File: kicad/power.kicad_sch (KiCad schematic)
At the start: 21 parts, among them U1 HT7533-1, U2 TLV62569DBV, U3 MCP6001T-E/OT

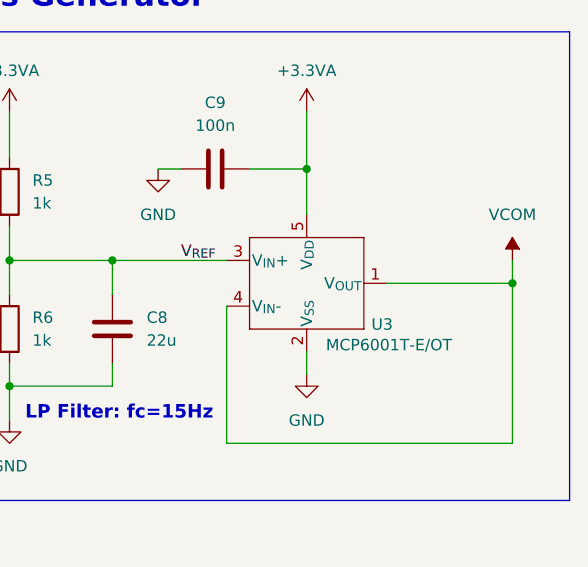
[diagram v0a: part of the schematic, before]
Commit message: Small update
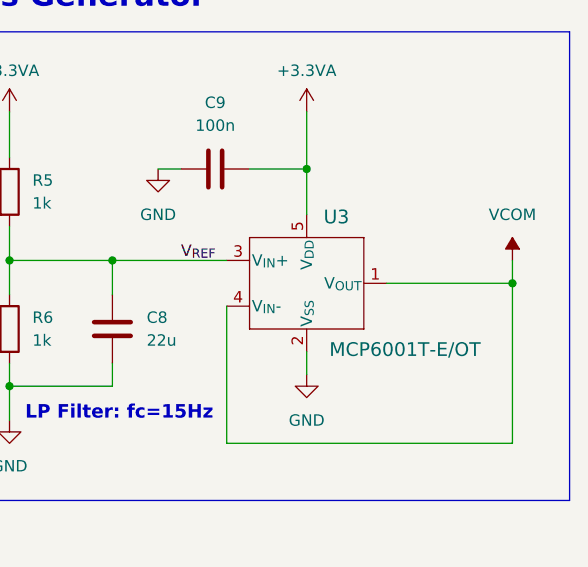
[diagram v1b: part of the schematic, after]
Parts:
- removed U3: MCP6001T-E/OT, SOT-23-5_MC_MCH, symbol bias_generator_ic:MCP6001T-E_OT
- added U3: MCP6001T-E/OT, SOT-23-5_MC_MCH, symbol bias_generator_microchip:MCP6001T-E_OT
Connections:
- net +3.3VA: now also U3.5 (V_{DD})
- net GND: now also U3.2 (V_{SS})
- net VCOM: now also U3.1 (V_{OUT}), U3.4 (V_{IN}-)
- net V_{REF}: now also U3.3 (V_{IN}+)
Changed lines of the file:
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@@
+	)
+	(symbol
+		(lib_id "bias_generator_microchip:MCP6001T-E_OT")
+		(at 229.87 63.5 0)
+		(unit 1)
+		(exclude_from_sim no)
+		(in_bom yes)
+		(on_board yes)
+		(dnp no)
+		(property "Reference" "U3"
+			(at 250.952 61.214 0)
+			(effects
+				(font
+					(size 1.524 1.524)
+				)
+			)
+		)
+		(property "Value" "MCP6001T-E/OT"
+			(at 258.572 75.946 0)
+			(effects
+				(font
+					(size 1.524 1.524)
+				)
+			)
+		)
+		(property "Footprint" "SOT-23-5_MC_MCH"
+			(at 232.918 53.086 0)
+			(effects
+				(font
+					(size 1.27 1.27)
+					(italic yes)
+				)
+				(hide yes)
+			)
+		)
+		(property "Datasheet" "MCP6001T-E/OT"
+			(at 233.934 56.134 0)
+			(effects
+				(font
+					(size 1.27 1.27)
+					(italic yes)
+				)
+				(hide yes)
+			)
+		)
+		(property "Description" ""
+			(at 229.87 63.5 0)
+			(effects
+				(font
+					(size 1.27 1.27)
+				)
+				(hide yes)
+			)
+		)
+		(pin "4"
+		)
+		(pin "5"
+		)
+		(pin "2"
+		)
+		(pin "1"
+		)
+		(pin "3"
+		)
+		(instances
+			(project ""
+				(path "/eba96202-8ea2-41d9-8d7a-700a4166585a/9e6a3319-b22e-494d-bd14-b1d6263414e0"
+					(reference "U3")
+					(unit 1)
+				)
+			)
+		)
 	)
 	(symbol
@@
 					(unit 1)
 				)
-			)
-		)
-	)
-	(symbol
-		(lib_id "bias_generator_ic:MCP6001T-E_OT")
-		(at 229.87 63.5 0)
-		(unit 1)
-		(exclude_from_sim no)
-		(in_bom yes)
-		(on_board yes)
-		(dnp no)
-		(property "Reference" "U3"
-			(at 256.032 73.152 0)
-			(effects
-				(font
-					(size 1.27 1.27)
-				)
-			)
-		)
-		(property "Value" "MCP6001T-E/OT"
-			(at 256.794 75.438 0)
-			(effects
-				(font
-					(size 1.27 1.27)
-				)
-			)
-		)
-		(property "Footprint" "SOT-23-5_MC_MCH"
-			(at 232.918 53.086 0)
-			(effects
-				(font
-					(size 1.27 1.27)
-					(italic yes)
-				)
-				(hide yes)
-			)
-		)
-		(property "Datasheet" "MCP6001T-E/OT"
-			(at 233.934 56.134 0)
-			(effects
-				(font
-					(size 1.27 1.27)
-					(italic yes)
-				)
-				(hide yes)
-			)
-		)
-		(property "Description" ""
-			(at 229.87 63.5 0)
-			(effects
-				(font
-					(size 1.27 1.27)
-				)
-				(hide yes)
-			)
-		)
-		(pin "5"
-		)
-		(pin "4"
-		)
-		(pin "3"
-		)
-		(pin "1"
-		)
-		(pin "2"
-		)
-		(instances
-			(project ""
-				(path "/eba96202-8ea2-41d9-8d7a-700a4166585a/9e6a3319-b22e-494d-bd14-b1d6263414e0"
-					(reference "U3")
-					(unit 1)
-				)
